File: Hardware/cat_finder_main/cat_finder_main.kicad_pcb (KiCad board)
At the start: 2 copper layers, 85 x 70 mm, 38 parts, among them J1 BATT, J10 Analog, J2 BME280, J3 CSS811, J4 DRIVERS, J5 GY-87, J7 FTDI, J8 Digital, U1 LD1117A33, U2 MCP732831CHARGER, U3 ESP32-CAM

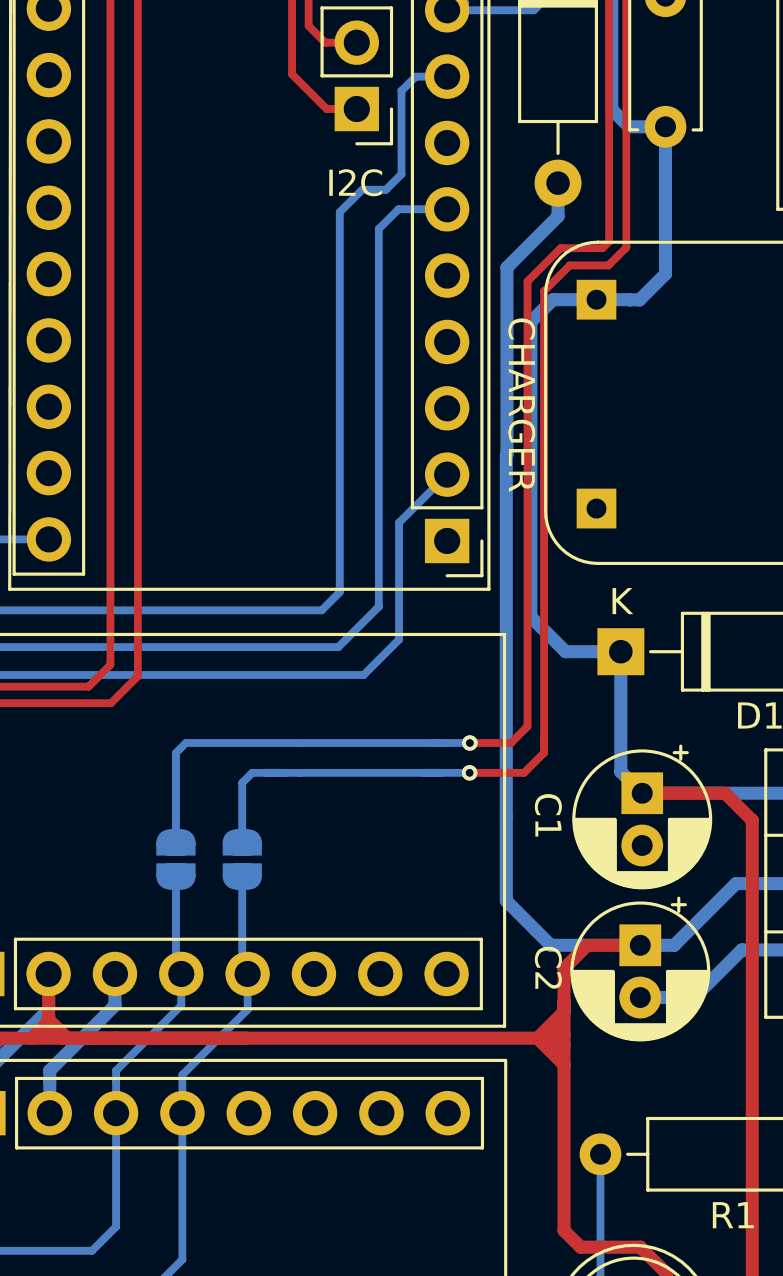
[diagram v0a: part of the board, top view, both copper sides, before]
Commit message: clone other repo
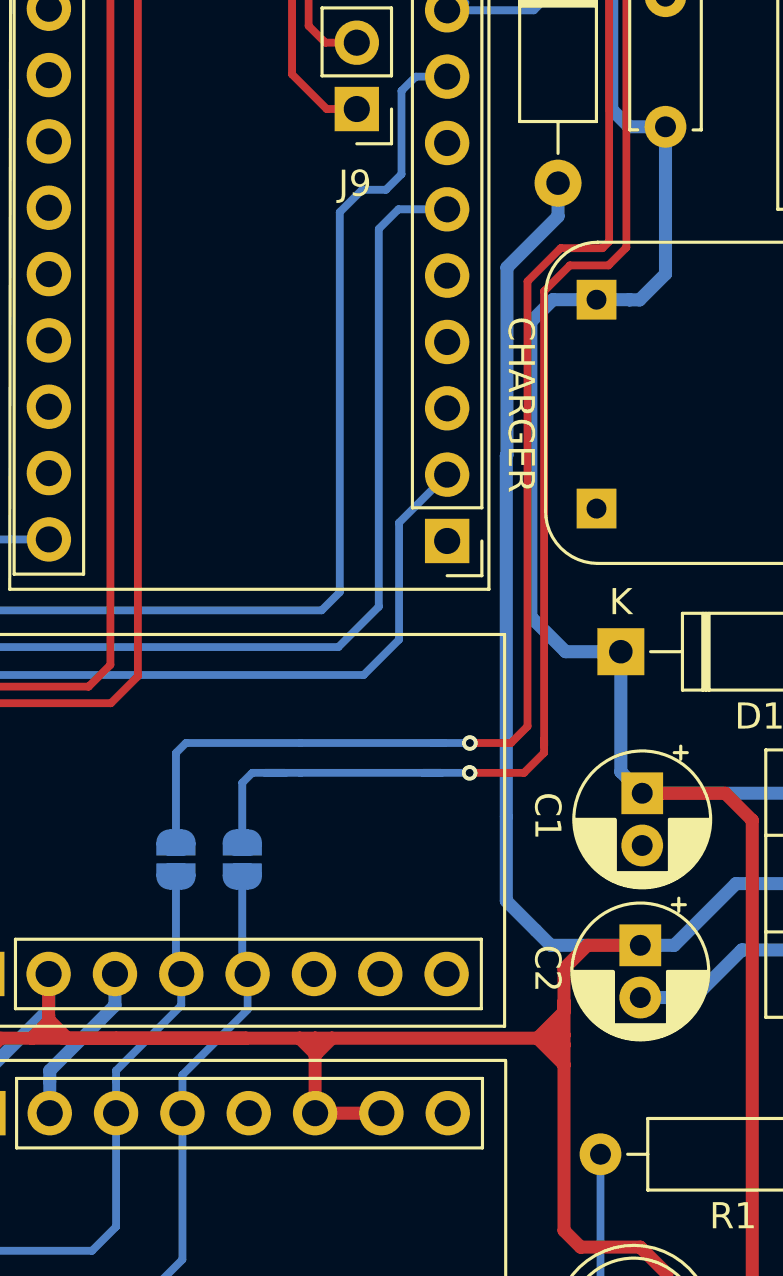
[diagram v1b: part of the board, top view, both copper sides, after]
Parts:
- renumbered SDA to J6, I2C to J9
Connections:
- J3 pad 5: /WAKE -> GND
- J3 pad 6: /INTCSS -> +3V3
- J3 pad 7: /RESET -> +3V3
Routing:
- net +3V3: track 170.8 -> 177.9 mm
